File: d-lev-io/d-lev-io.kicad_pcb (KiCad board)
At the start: 4 copper layers, 125 x 50.1 mm, 141 parts, among them IC1 ES9010K2M, IC3 MAX97220C/MAX97220D, J1 USB_C_Receptacle_USB2.0, J2 PJ-059A, J3 Conn_01x12_MountingPin, J4 MIDI_OUT_JACK, J5 PROG_HDR, J6 HEADPHONE, J7 TOUCH_HDR, J8 CV_HDR, SW1 SW_Push, SW2 SW_Push, SW3 SW_Push, U1 ATSAMD11D14A-M, U2 TPS54202DDC, U3 ADP151-3.3, U4 74LVC2GU04, U5 AP2112K-3.3, U6 74AHC1G126, U7 USBLC6-2SC6, X1 7M-50.000MAAJ-T

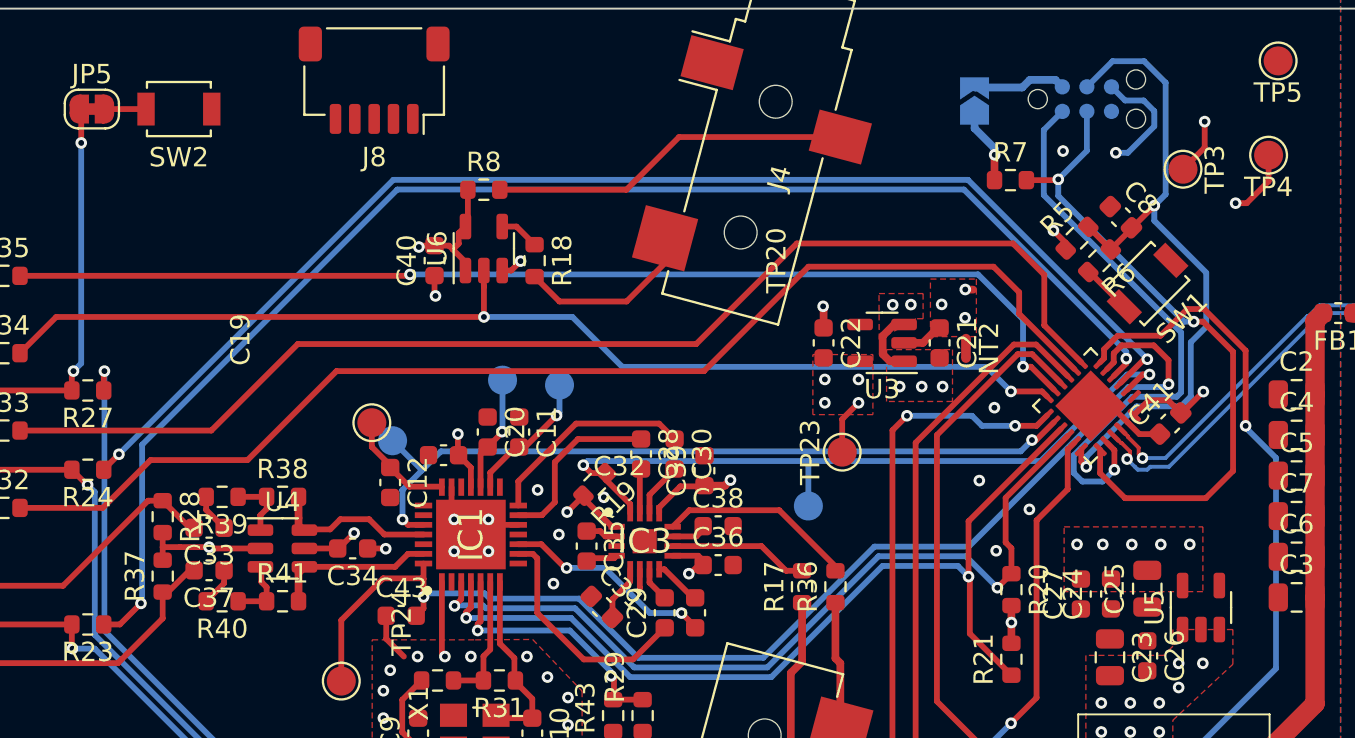
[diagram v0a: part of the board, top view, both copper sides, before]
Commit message: route cv header
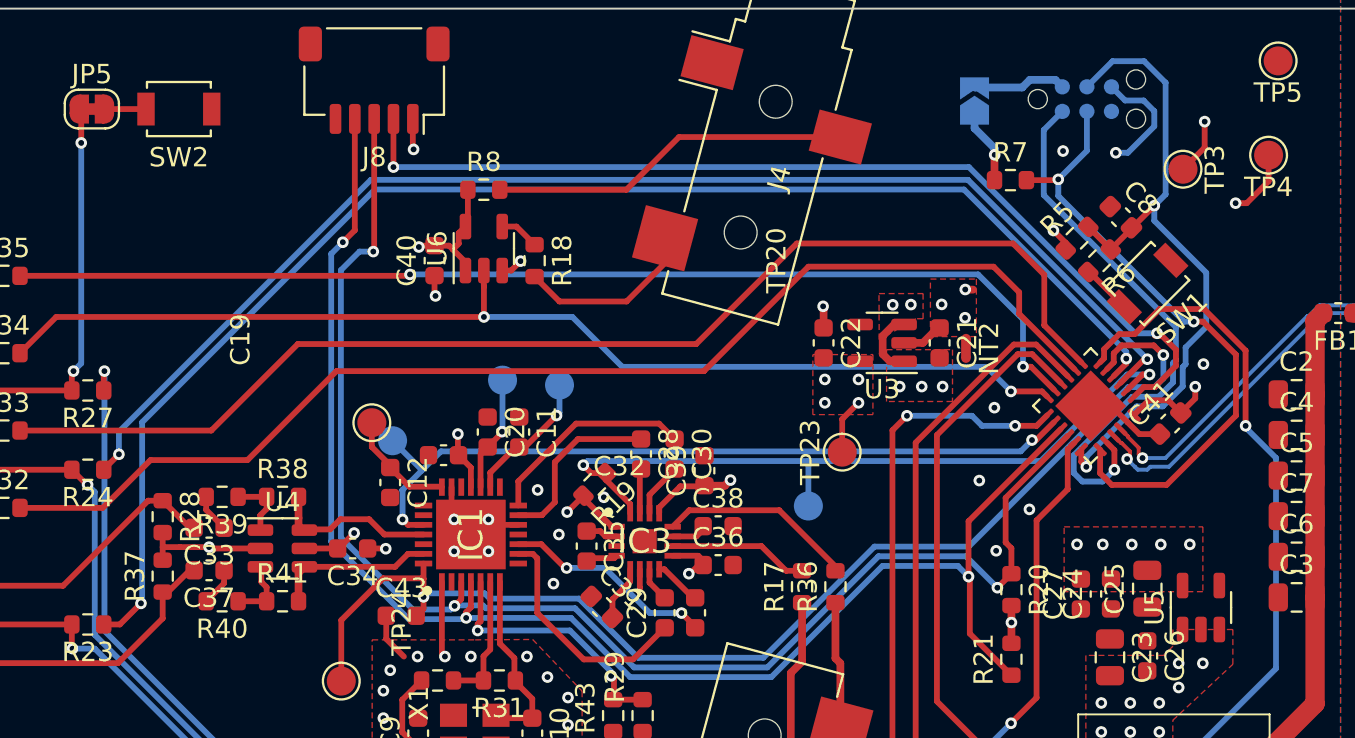
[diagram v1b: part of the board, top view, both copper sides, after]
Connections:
- J8 pad 3: /DAC/SDA -> /DAC/SCL
- J8 pad 4: /DAC/SCL -> /DAC/SDA
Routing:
- net /SAMD11/CV_EN: track 0.00 -> 50.6 mm, vias 0 -> 2
- net /DAC/SDA: track 47.4 -> 78.5 mm, vias 2 -> 3
- net /DAC/SCL: track 43.5 -> 73.7 mm, vias 2 -> 3
- net /SAMD11/JTAG.SWCLK: track 34.4 -> 32.4 mm
- net VDD: track 17.3 -> 18.9 mm, vias 17 -> 18
- net /SAMD11/JTAG.SWDIO: track 29.8 -> 29.0 mm
- net Net-(U1-PA05): track 72.0 -> 72.6 mm
- net Net-(U1-PA04): track 65.9 -> 66.6 mm
- net /DAC/DAC_RESET: track 62.5 -> 62.0 mm
- net /SAMD11/~{RST}: track 36.1 -> 35.6 mm
- net GND: vias 61 -> 62
